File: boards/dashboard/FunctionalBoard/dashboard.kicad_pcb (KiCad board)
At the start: 2 copper layers, 79.1 x 34.2 mm, 43 parts, among them IC1 ATMEGA16M1, J1 micromatch_male_10, J2 micromatch_male_14, J3 micromatch_female_RA_6, P1 CONN_02X03, U1 CAN_Transceiver, U2 TPS561201, U3 LM3480, U4 CP2120, Y1 Crystal_SMD

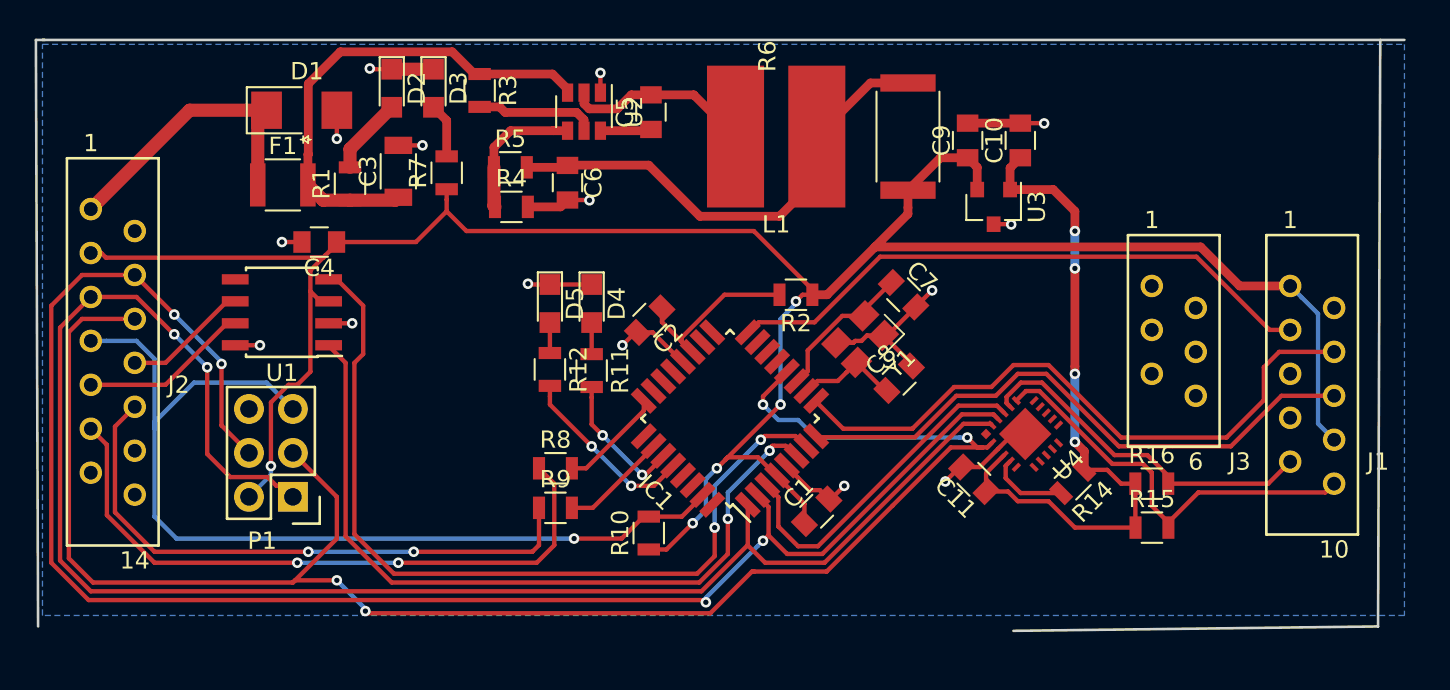
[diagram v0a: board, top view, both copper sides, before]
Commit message: Gerber and BOM files for functional board
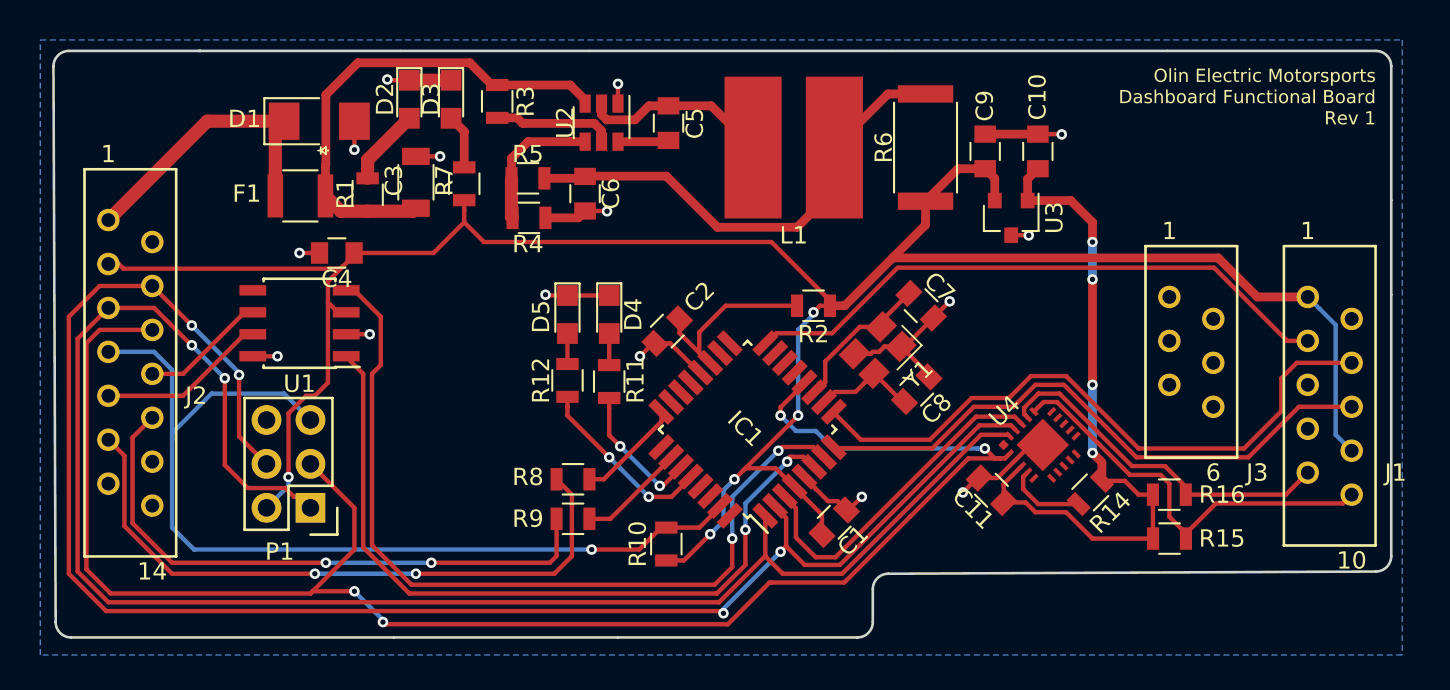
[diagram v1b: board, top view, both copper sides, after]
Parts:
- moved C7 1.20 mm to (169.0, 54.7)
- moved R3 1.20 mm to (144.5, 42.9)
- moved C10 1.20 mm to (175.8, 45.8)
- moved C9 1.20 mm to (172.7, 45.8)
- moved D3 1.20 mm to (141.9, 42.8)
- moved J1 1.20 mm to (191.4, 59.3)
- moved R4 1.20 mm to (146.4, 49.7)
- moved R7 1.20 mm to (142.6, 47.7)
- moved U2 1.20 mm to (150.6, 44.2)
- moved R10 1.20 mm to (154.3, 68.5)
- moved C11 1.20 mm to (173.1, 65.4)
- moved C2 1.20 mm to (154.4, 56.2)
- moved C8 1.20 mm to (168.8, 59.6)
- moved D1 1.20 mm to (134.2, 44.1)
- moved IC1 1.20 mm to (159.0, 61.9)
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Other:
- board size 79.1 x 34.2 mm -> 77.3 x 33.9 mm
- board text added: "Olin Electric Motorsports Dashboard Functional Board Rev 1"
